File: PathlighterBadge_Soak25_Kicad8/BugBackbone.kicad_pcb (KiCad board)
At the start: 2 copper layers, 21.7 x 75.4 mm, 3 parts

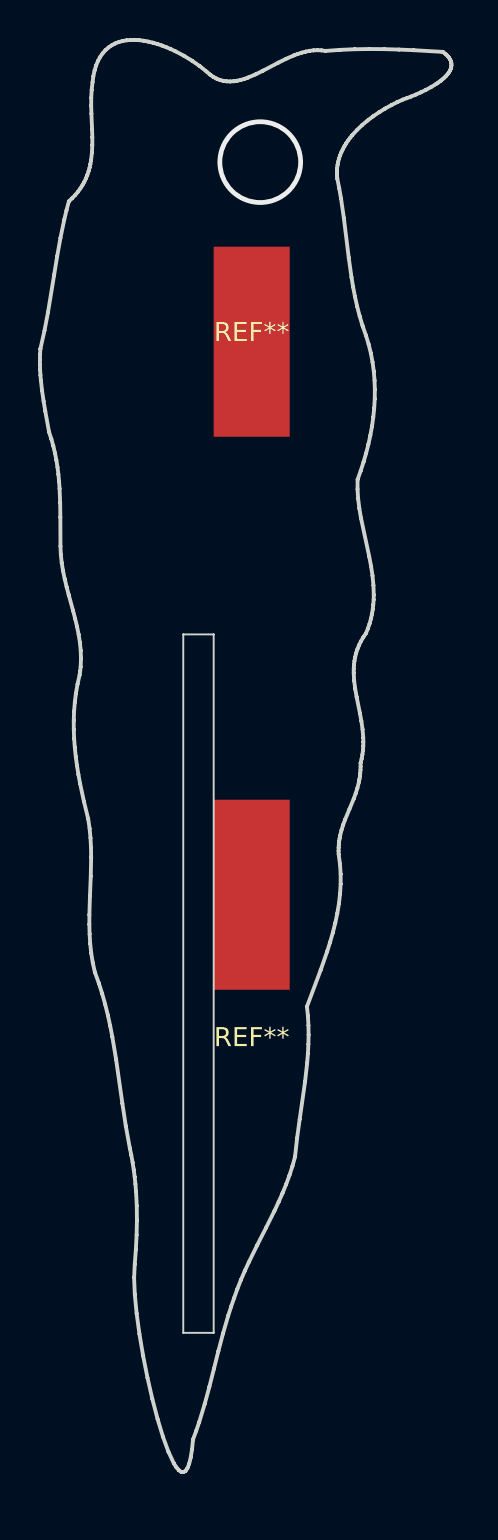
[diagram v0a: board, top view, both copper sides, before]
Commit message: Rework backbone
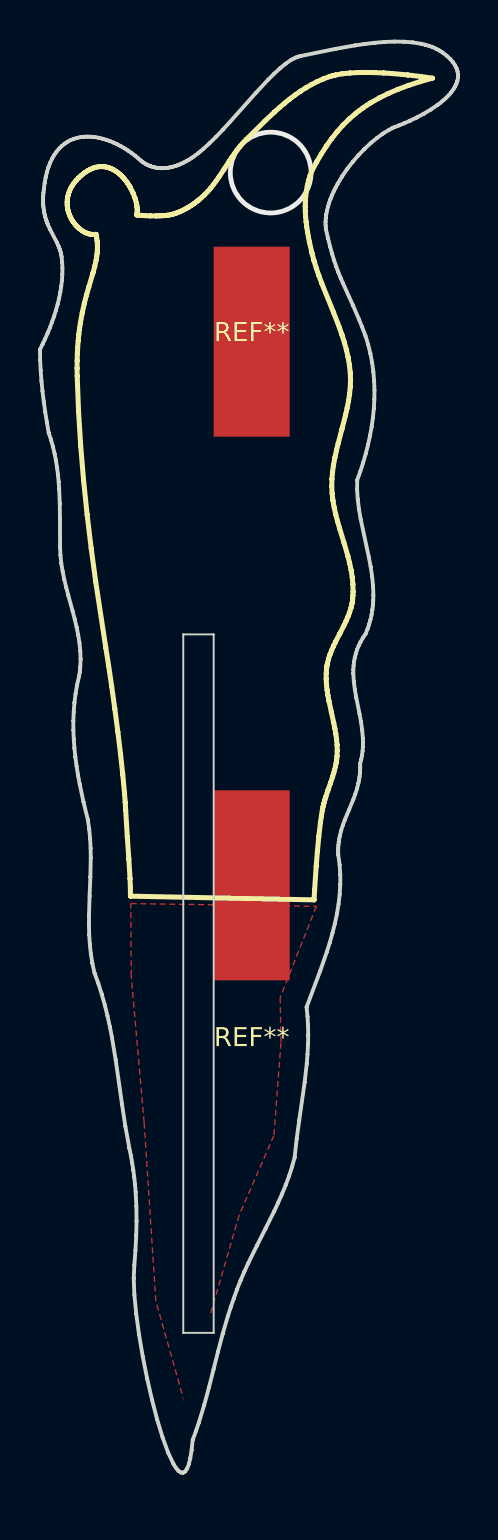
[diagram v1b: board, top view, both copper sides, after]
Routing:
- added copper zone on F.Cu, net (none)
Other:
- board size 21.7 x 75.4 mm -> 22 x 75.3 mm
